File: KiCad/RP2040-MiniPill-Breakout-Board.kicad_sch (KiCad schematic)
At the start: 11 parts, among them J1 Conn_01x20_Socket, J2 Conn_01x20_Socket, J3 Screw_Terminal_01x20, J4 Screw_Terminal_01x20, U1 TPS3700

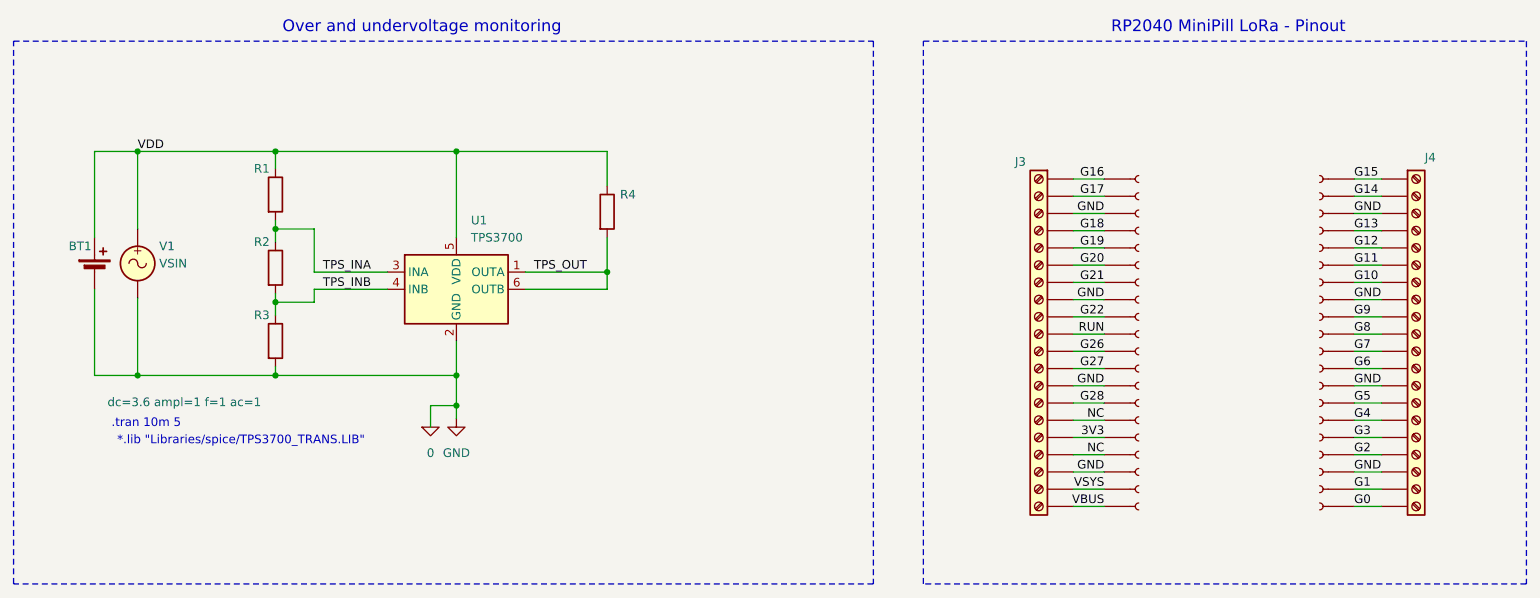
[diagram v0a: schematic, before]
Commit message: adding Simulation
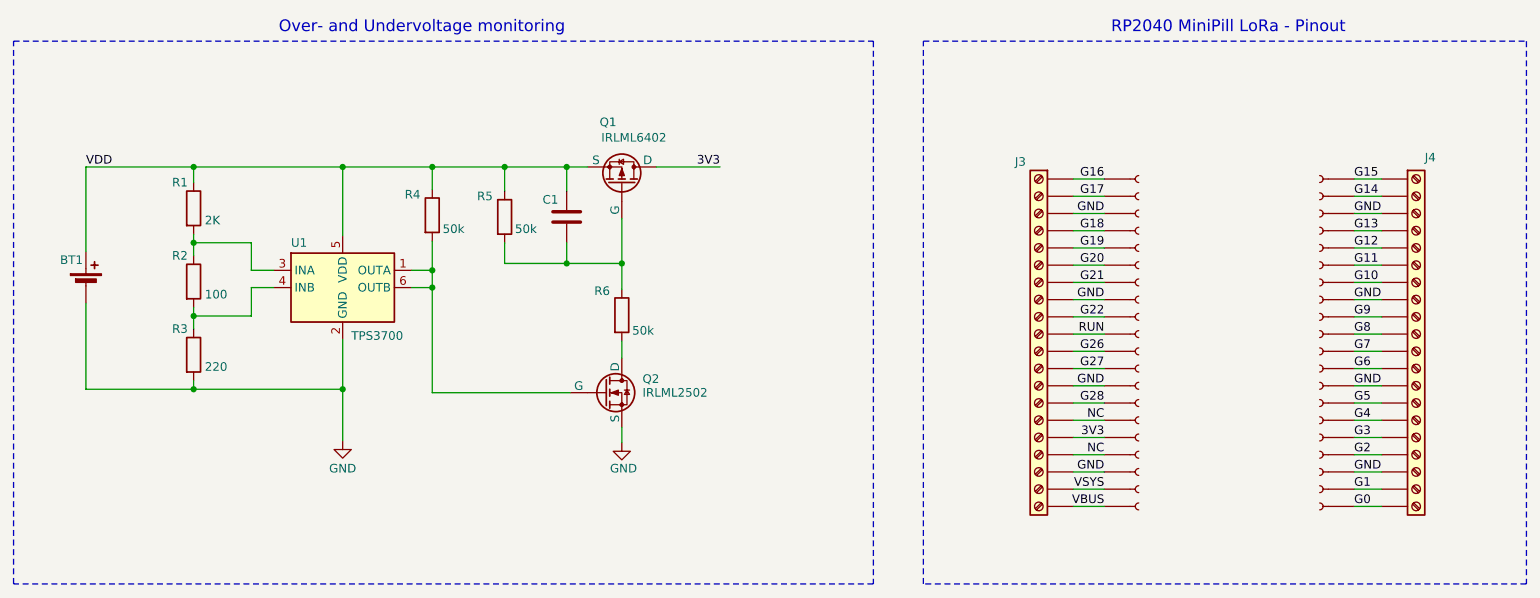
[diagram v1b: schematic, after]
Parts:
- removed V1: VSIN, symbol Simulation_SPICE:VSIN
- added C1: C, Capacitor_SMD:C_0603_1608Metric_Pad1.08x0.95mm_HandSolder, symbol Device:C
- added Q1: IRLML6402, Package_TO_SOT_SMD:SOT-23, symbol Device:Q_PMOS
- added Q2: IRLML2502, Package_TO_SOT_SMD:SOT-23, symbol Device:Q_NMOS
- added R5, R6: 50k, Resistor_SMD:R_0603_1608Metric_Pad0.98x0.95mm_HandSolder, symbol Device:R
- R1: value ${SIM.PARAMS} -> 2K; footprint (none) -> Resistor_SMD:R_0603_1608Metric_Pad0.98x0.95mm_HandSolder
- R2: value ${SIM.PARAMS} -> 100; footprint (none) -> Resistor_SMD:R_0603_1608Metric_Pad0.98x0.95mm_HandSolder
- R3: value ${SIM.PARAMS} -> 220; footprint (none) -> Resistor_SMD:R_0603_1608Metric_Pad0.98x0.95mm_HandSolder
- R4: value ${SIM.PARAMS} -> 50k; footprint (none) -> Resistor_SMD:R_0603_1608Metric_Pad0.98x0.95mm_HandSolder
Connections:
- net 3V3: now also Q1.D
- net VDD: now also C1.1, Q1.S, R5.1
- net 0 renamed GND
- net GND: now also Q2.S
- net TPS_INA: no longer names the net of R1.2, R2.1, U1.3 (INA)
- net TPS_INB: no longer names the net of R2.2, R3.1, U1.4 (INB)
- net TPS_OUT: no longer names the net of R4.2, U1.1 (OUTA), U1.6 (OUTB)
- net TPS_OUT: now also Q2.G
- new net: C1.2, Q1.G, R5.2, R6.1
- new net: Q2.D, R6.2
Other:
- note added: "Over- and Undervoltage monitoring"
- note removed: "*.lib "Libraries/spice/TPS3700_TRANS.LIB""
- note removed: ".tran 10m 5"
- note removed: "Over and undervoltage monitoring"
- title: (none) -> RP2040-MiniPill-Breakout-Board
- moved on the sheet: BT1, R1, R2, R3, R4, U1
